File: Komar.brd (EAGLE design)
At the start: 58 x 58 mm, 107 parts, among them CON1 USB-VERTICAL, CON2 PINHEAD_1X01-2, CON3 CON-4P-TABS-STRAIGHT, CON4 CON-4P-TABS-STRAIGHT, CON5 CON-4P-TABS-STRAIGHT, CON6 CON-4P-TABS-STRAIGHT, CON7 CON-4P-TABS-STRAIGHT, CON8 CON-6P-SM06B, CON9 PINHEAD_1X01-2, IC1 TPD3S014DBVR-SOT23-6, IC2 TPD3S014DBVR-SOT23-6, IC3 ATA6561-GBQW-N-HVSON8, IC4 ATA6561-GBQW-N-HVSON8, IC5 MCP9700AT-E/TTVAO-SOT23, IC6 11LC040T-E/TT, Q1 FDMS86368-F085, Q10 FDMS86368-F085, Q11 FDMS86368-F085, Q12 FDMS86368-F085, Q2 FDMS86368-F085, Q3 FDMS86368-F085, Q4 FDMS86368-F085, Q5 FDMS86368-F085, Q6 FDMS86368-F085, Q7 FDMS86368-F085, Q8 FDMS86368-F085, Q9 FDMS86368-F085

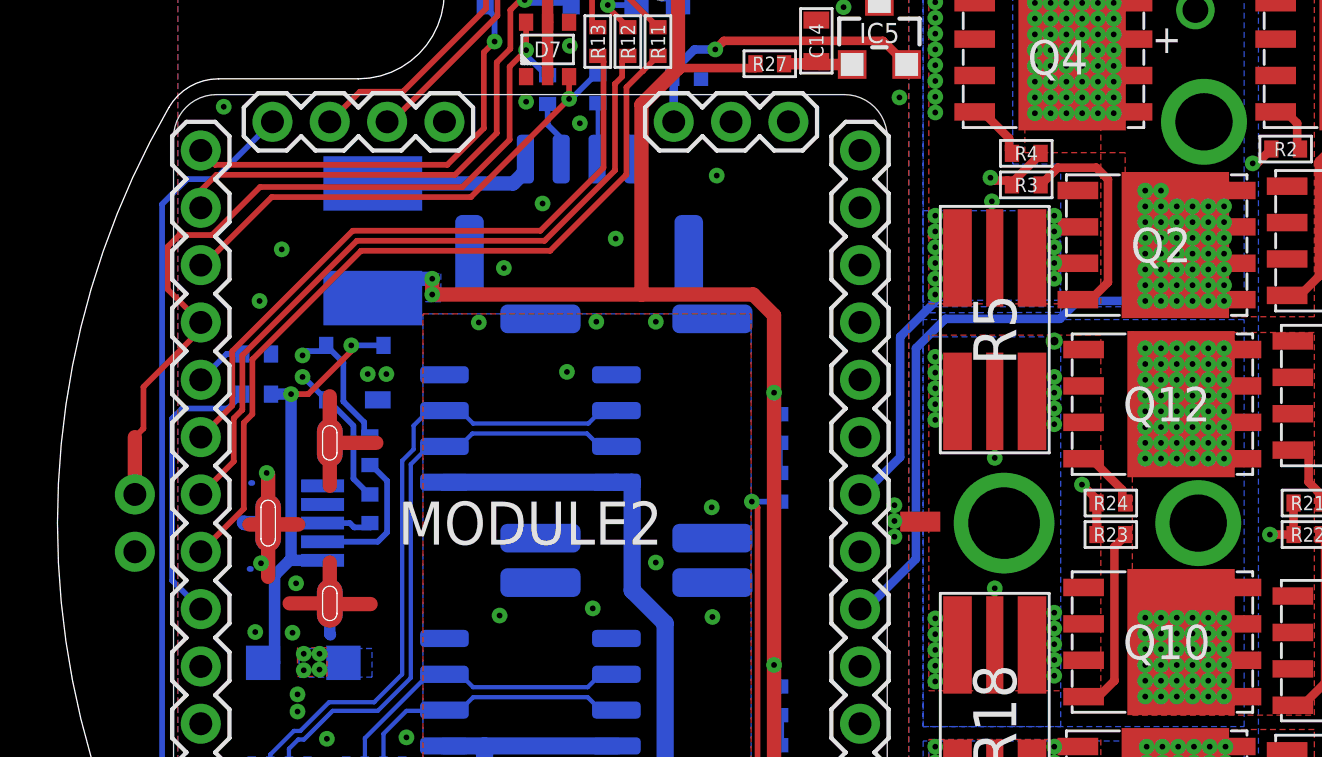
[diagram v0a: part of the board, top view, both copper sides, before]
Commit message: width updates
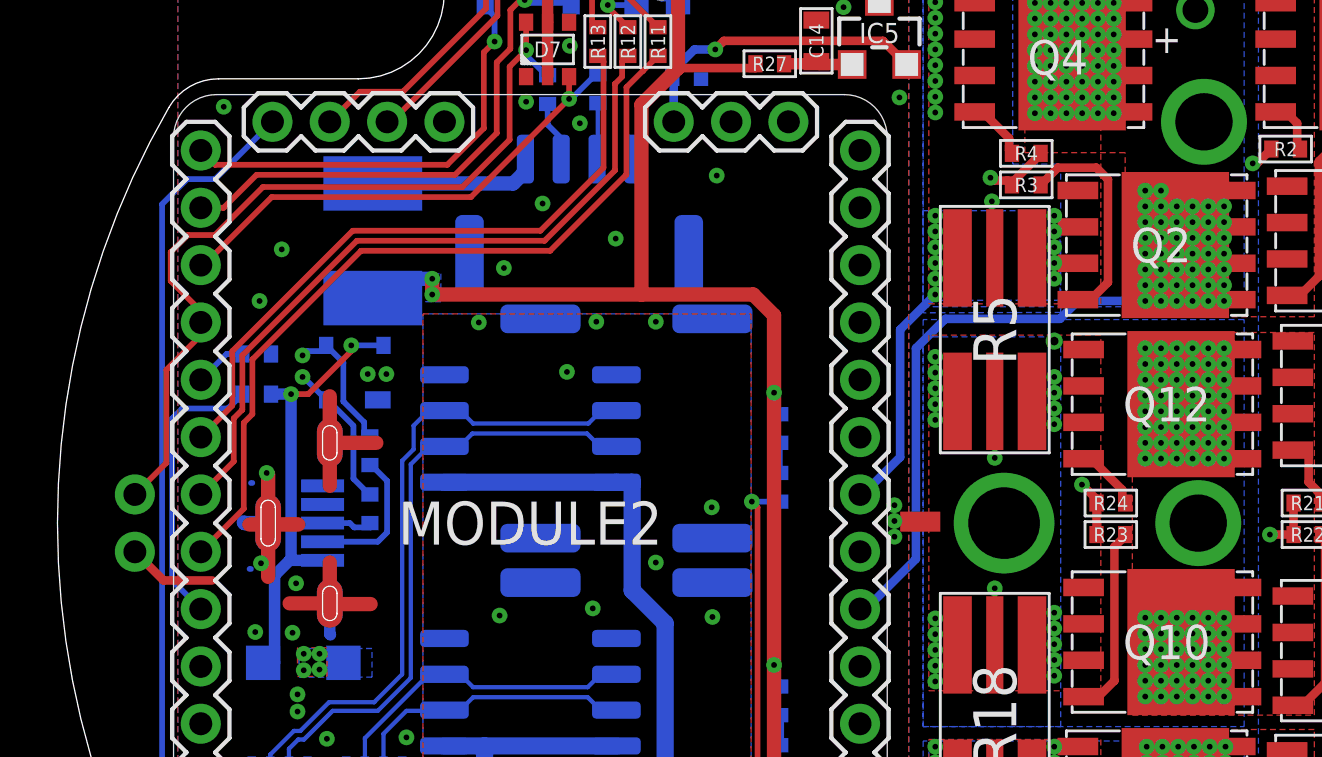
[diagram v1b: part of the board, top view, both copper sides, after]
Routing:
- net GND: track 33.8 -> 36.9 mm
- net PHASE_C: track 15.7 -> 15.1 mm
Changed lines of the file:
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@@
 <setting verticaltext="up"/>
 </settings>
-<grid distance="0.1" unitdist="mm" unit="mm" style="lines" multiple="1" display="yes" altdistance="0.1" altunitdist="mm" altunit="mm"/>
+<grid distance="1" unitdist="mm" unit="mm" style="lines" multiple="1" display="yes" altdistance="0.1" altunitdist="mm" altunit="mm"/>
 <layers>
-<layer number="1" name="Top" color="4" fill="1" visible="no" active="yes"/>
+<layer number="1" name="Top" color="4" fill="1" visible="yes" active="yes"/>
 <layer number="2" name="Route2" color="1" fill="3" visible="no" active="yes"/>
 <layer number="3" name="Route3" color="4" fill="3" visible="no" active="yes"/>
@@
 <layer number="19" name="Unrouted" color="6" fill="1" visible="yes" active="yes"/>
 <layer number="20" name="Dimension" color="24" fill="1" visible="yes" active="yes"/>
-<layer number="21" name="tPlace" color="7" fill="1" visible="no" active="yes"/>
+<layer number="21" name="tPlace" color="7" fill="1" visible="yes" active="yes"/>
 <layer number="22" name="bPlace" color="7" fill="1" visible="yes" active="yes"/>
-<layer number="23" name="tOrigins" color="15" fill="1" visible="no" active="yes"/>
+<layer number="23" name="tOrigins" color="15" fill="1" visible="yes" active="yes"/>
 <layer number="24" name="bOrigins" color="15" fill="1" visible="yes" active="yes"/>
-<layer number="25" name="tNames" color="7" fill="1" visible="no" active="yes"/>
+<layer number="25" name="tNames" color="7" fill="1" visible="yes" active="yes"/>
 <layer number="26" name="bNames" color="7" fill="1" visible="yes" active="yes"/>
 <layer number="27" name="tValues" color="7" fill="1" visible="no" active="yes"/>
@@
 <layer number="49" name="Reference" color="7" fill="1" visible="no" active="yes"/>
 <layer number="50" name="dxf" color="7" fill="1" visible="no" active="no"/>
-<layer number="51" name="tDocu" color="7" fill="1" visible="no" active="yes"/>
+<layer number="51" name="tDocu" color="7" fill="1" visible="yes" active="yes"/>
 <layer number="52" name="bDocu" color="7" fill="1" visible="yes" active="yes"/>
 <layer number="53" name="tGND_GNDA" color="7" fill="9" visible="no" active="no"/>
@@
 <via x="12.7" y="14.15" extent="1-16" drill="0.2" diameter="0.55"/>
 <via x="8.15" y="16.1" extent="1-16" drill="0.2" diameter="0.55"/>
+<wire x1="2.7" y1="28" x2="3.7" y2="27" width="0.3" layer="1"/>
+<wire x1="3.7" y1="27" x2="5.4" y2="27" width="0.3" layer="1"/>
 <wire x1="9.5" y1="31.8" x2="9.5" y2="31.8" width="0" layer="19" extent="1-16"/>
 <wire x1="9.35" y1="31.8" x2="9.5" y2="31.8" width="0" layer="19" extent="1-1"/>
-<wire x1="2.7" y1="28" x2="6.5" y2="29.025" width="0" layer="19" extent="16-16"/>
 </signal>
 <signal name="PHASE_A_GND">
@@
 <contactref element="MODULE2" pad="8"/>
 <via x="30.625" y="39.175" extent="1-16" drill="0.2" diameter="0.55"/>
-<wire x1="30.45" y1="39" x2="30.625" y2="39.175" width="0.2" layer="1"/>
 <wire x1="28" y1="30" x2="28.1" y2="30" width="0.3" layer="16"/>
 <wire x1="28.1" y1="30" x2="29.4" y2="31.3" width="0.3" layer="16"/>
-<wire x1="29.4" y1="31.3" x2="29.4" y2="35.50281875" width="0.3" layer="16"/>
-<wire x1="29.4" y1="35.50281875" x2="30.625" y2="36.72781875" width="0.3" layer="16"/>
+<wire x1="29.4" y1="35.75" x2="30.625" y2="36.975" width="0.3" layer="16"/>
+<wire x1="29.4" y1="31.3" x2="29.4" y2="35.75" width="0.3" layer="16"/>
 </signal>
 <signal name="PHASE_B_CURRENT_SHUNT_N">
@@
 <contactref element="Q10" pad="8"/>
 <contactref element="Q10" pad="P$1"/>
-<wire x1="37.5" y1="35.55" x2="37.95" y2="35.1" width="0.3" layer="1"/>
 <wire x1="28" y1="34" x2="26.95" y2="35.05" width="0.2" layer="15"/>
 <wire x1="26.95" y1="35.05" x2="26.95" y2="36.29350625" width="0.2" layer="15"/>
@@
 <contactref element="D7" pad="6"/>
 <contactref element="CON2" pad="1"/>
-<wire x1="2.7" y1="30" x2="2.7" y2="32" width="0.5" layer="1"/>
 <via x="16.35" y="45.5" extent="1-16" drill="0.2" diameter="0.55"/>
 <wire x1="16.35" y1="45.5" x2="16.35" y2="46.475" width="0.2" layer="1"/>
@@
 <wire x1="15.775" y1="44.925" x2="15.775" y2="42.375" width="0.2" layer="1"/>
 <contactref element="MODULE2" pad="25"/>
-<wire x1="5" y1="36" x2="5" y2="35.75" width="0.2" layer="1"/>
-<wire x1="5" y1="35.75" x2="3" y2="33.75" width="0.2" layer="1"/>
-<wire x1="3" y1="33.75" x2="3" y2="32.3" width="0.2" layer="1"/>
-<wire x1="3" y1="32.3" x2="2.7" y2="32" width="0.2" layer="1"/>
-<wire x1="5.39350625" y1="39.05" x2="4.25" y2="39.05" width="0.2" layer="1"/>
-<wire x1="7.06850625" y1="40.725" x2="5.39350625" y2="39.05" width="0.2" layer="1"/>
-<wire x1="4.25" y1="39.05" x2="3.85" y2="38.65" width="0.2" layer="1"/>
-<wire x1="3.85" y1="37.15" x2="5" y2="36" width="0.2" layer="1"/>
-<wire x1="14.125" y1="40.725" x2="7.06850625" y2="40.725" width="0.2" layer="1"/>
-<wire x1="3.85" y1="38.65" x2="3.85" y2="37.15" width="0.2" layer="1"/>
+<wire x1="5" y1="36" x2="5" y2="35.55" width="0.2" layer="1"/>
+<wire x1="5" y1="35.55" x2="3.8" y2="34.35" width="0.2" layer="1"/>
+<wire x1="5.49350625" y1="39.05" x2="4.55" y2="39.05" width="0.2" layer="1"/>
+<wire x1="7.16850625" y1="40.725" x2="5.49350625" y2="39.05" width="0.2" layer="1"/>
+<wire x1="4.55" y1="39.05" x2="3.95" y2="38.45" width="0.2" layer="1"/>
+<wire x1="5" y1="36.4" x2="5" y2="36" width="0.2" layer="1"/>
+<wire x1="5" y1="36.4" x2="3.95" y2="37.45" width="0.2" layer="1"/>
+<wire x1="14.125" y1="40.725" x2="7.16850625" y2="40.725" width="0.2" layer="1"/>
+<wire x1="3.95" y1="38.45" x2="3.95" y2="37.45" width="0.2" layer="1"/>
+<wire x1="3.8" y1="31.1" x2="2.7" y2="30" width="0.2" layer="1"/>
+<wire x1="3.8" y1="34.35" x2="3.8" y2="31.1" width="0.2" layer="1"/>
 </signal>
 <signal name="GAIN_OUT">
@@
 <signal name="GATE_ENABLE_OUT">
 <contactref element="LED4" pad="A"/>
-<wire x1="5.544975" y1="41.15" x2="13.869975" y2="41.15" width="0.2" layer="1"/>
-<wire x1="5" y1="40.605025" x2="5.544975" y2="41.15" width="0.2" layer="1"/>
+<wire x1="6.944975" y1="41.15" x2="13.869975" y2="41.15" width="0.2" layer="1"/>
+<wire x1="5" y1="40" x2="5.794975" y2="40" width="0.2" layer="1"/>
+<wire x1="6.944975" y1="41.15" x2="5.794975" y2="40" width="0.2" layer="1"/>
 <via x="16.3" y="47.25" extent="1-16" drill="0.2" diameter="0.55"/>
 <wire x1="13.869975" y1="41.15" x2="15.325" y2="42.605025" width="0.2" layer="1"/>
@@
 <wire x1="16.4" y1="47.15" x2="17.775" y2="47.15" width="0.2" layer="16"/>
 <contactref element="MODULE2" pad="23"/>
-<wire x1="5" y1="40" x2="5" y2="40.605025" width="0.2" layer="1"/>
 </signal>
 <signal name="UART_RX">
